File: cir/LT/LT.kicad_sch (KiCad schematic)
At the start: 24 parts, among them J1 Conn_01x04_Socket, J2 Conn_01x04_Socket, J3 Conn_01x02_Socket, U1 LBR-127HLD, U2 74HC7014, U4 LBR-127HLD, U5 LBR-127HLD, U6 LBR-127HLD

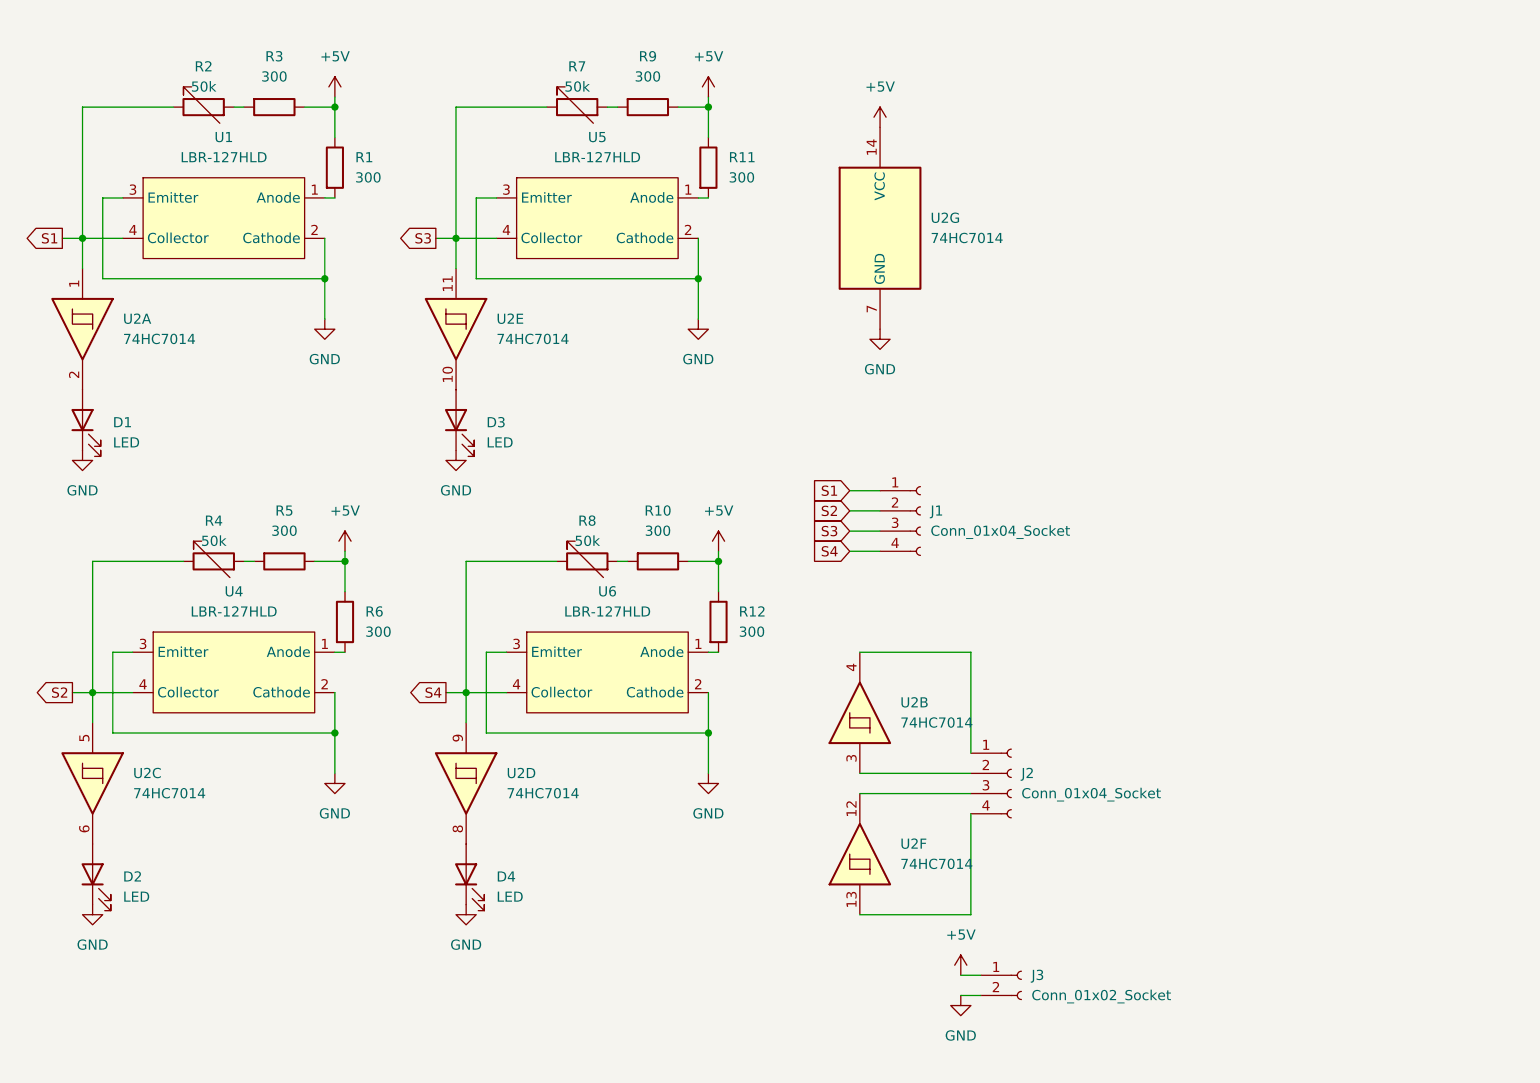
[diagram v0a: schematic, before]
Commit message: u
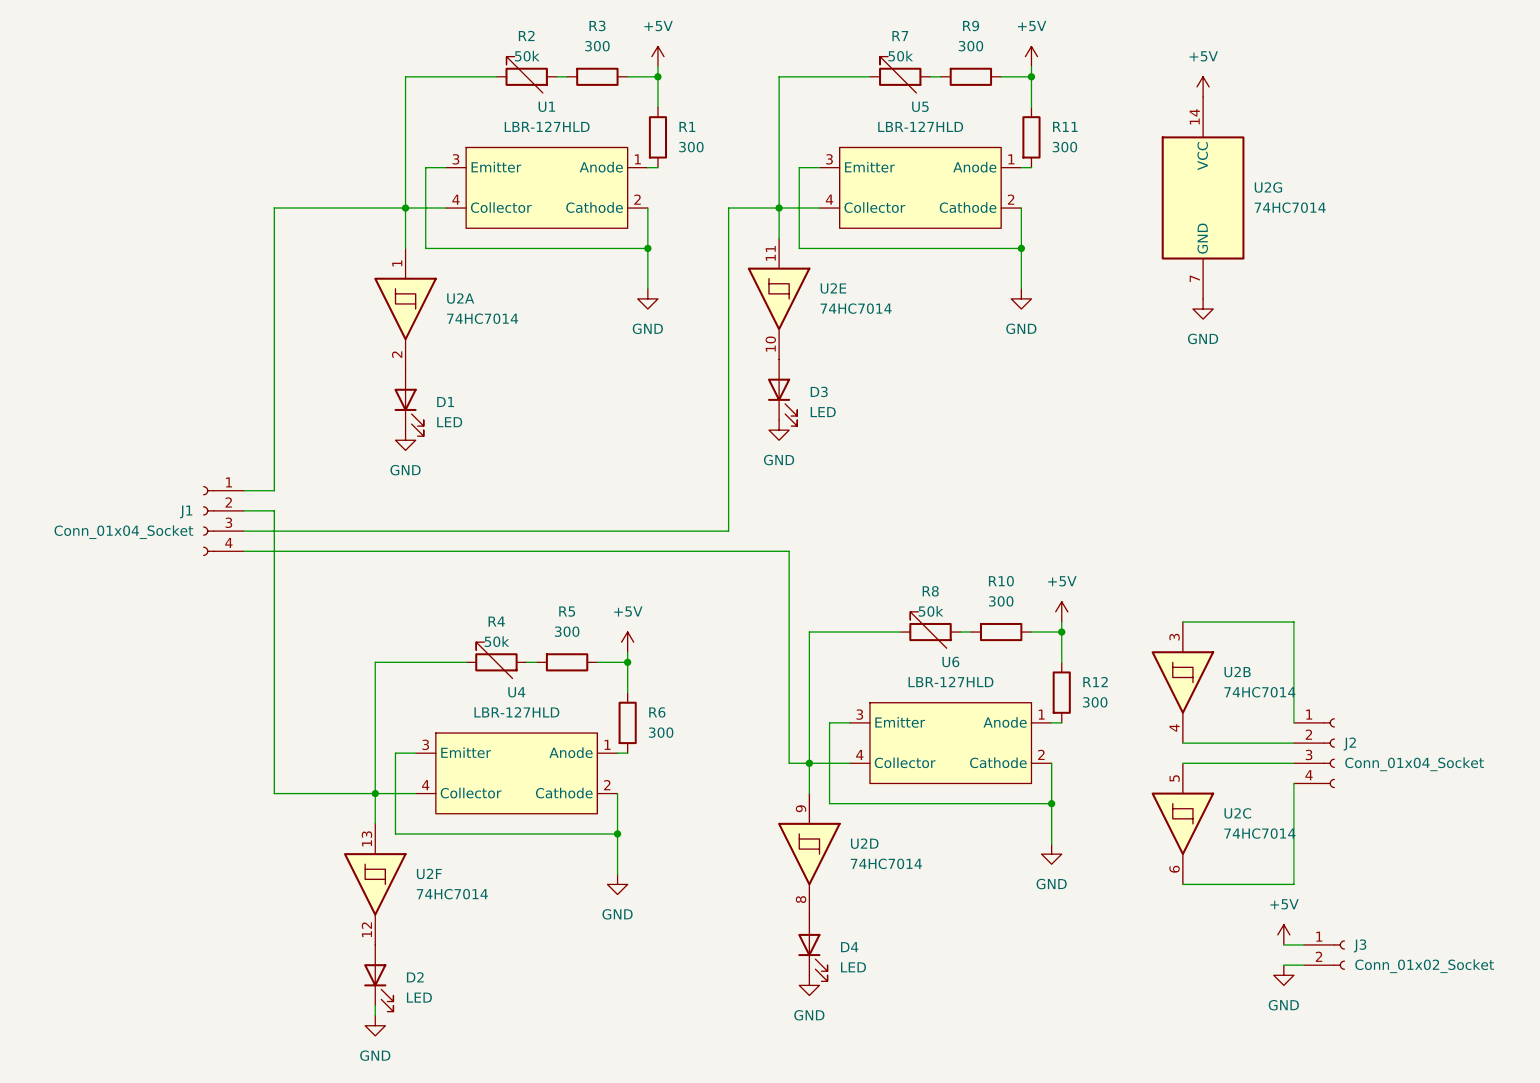
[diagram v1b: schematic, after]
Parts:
- R1, R10, R11, R12, R3, R5, R6, R9: footprint Resistor_SMD:R_2010_5025Metric -> Resistor_THT:R_Axial_DIN0204_L3.6mm_D1.6mm_P5.08mm_Horizontal
- U2: footprint Package_SO:SOIC-14_3.9x8.7mm_P1.27mm -> Package_DIP:DIP-14_W7.62mm_Socket
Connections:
- net at D2.2 (A): now also U2.12; no longer U2.6
- net at J2.1 (Pin_1): now also U2.3; no longer U2.4
- net at J2.2 (Pin_2): now also U2.4; no longer U2.3
- net at J2.3 (Pin_3): now also U2.5; no longer U2.12
- net at J2.4 (Pin_4): now also U2.6; no longer U2.13
- net S1: no longer names the net of J1.1 (Pin_1), R2.1, U1.4 (Collector), U2.1
- net S2: no longer names the net of J1.2 (Pin_2), R4.1, U4.4 (Collector)
- net S2: now also U2.13; no longer U2.5
- net S3: no longer names the net of J1.3 (Pin_3), R7.1, U2.11, U5.4 (Collector)
- net S4: no longer names the net of J1.4 (Pin_4), R8.1, U2.9, U6.4 (Collector)
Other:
- moved on the sheet: D1, D2, D3, D4, J1, J2, J3, R1, R10, R11, R12, R2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
